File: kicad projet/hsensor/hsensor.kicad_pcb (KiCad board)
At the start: 2 copper layers, 79.5 x 98 mm, 29 parts, among them J2_0 Conn_01x02_Pin, J2_1 Conn_01x02_Pin, J2_2 Conn_01x02_Pin, J3 Conn_01x03_Pin, U1 TLV75801PDBV, U2 TLV75801PDBV, U3 LM358

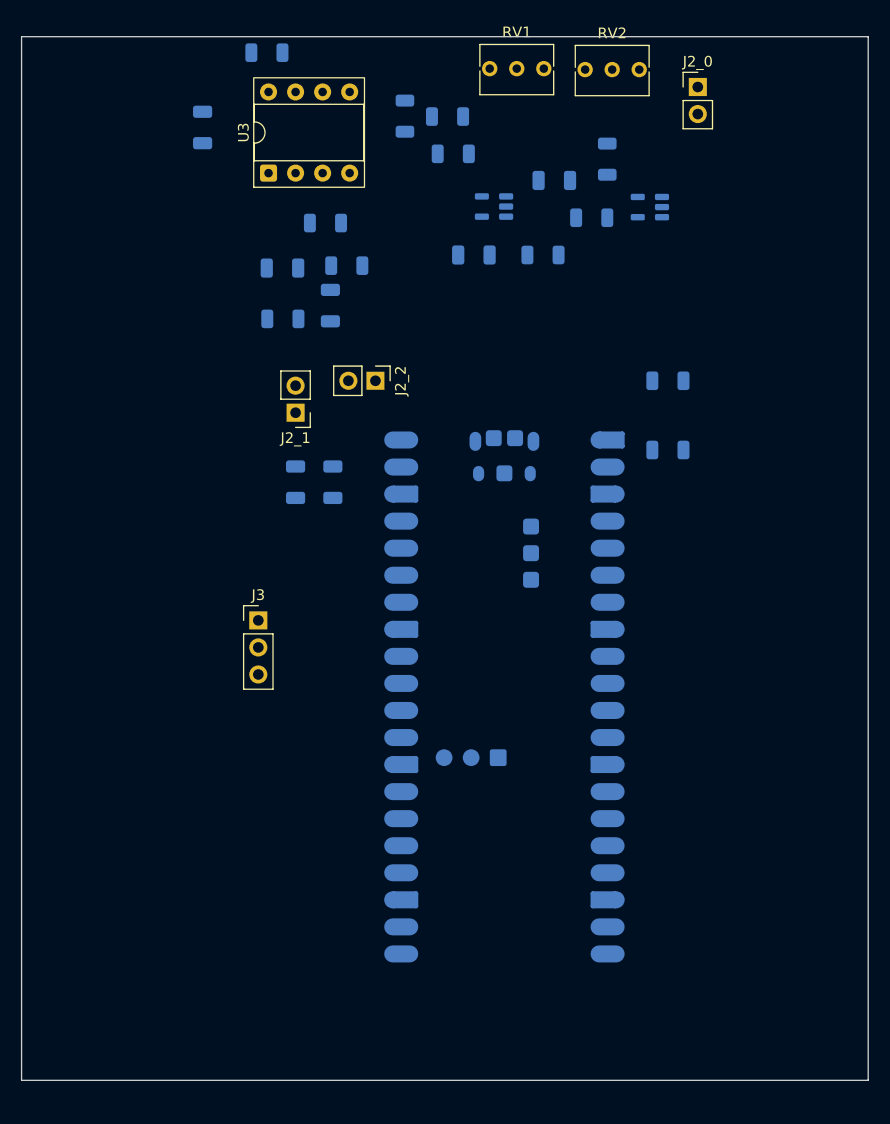
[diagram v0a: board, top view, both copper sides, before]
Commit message: final pcb (i hope)
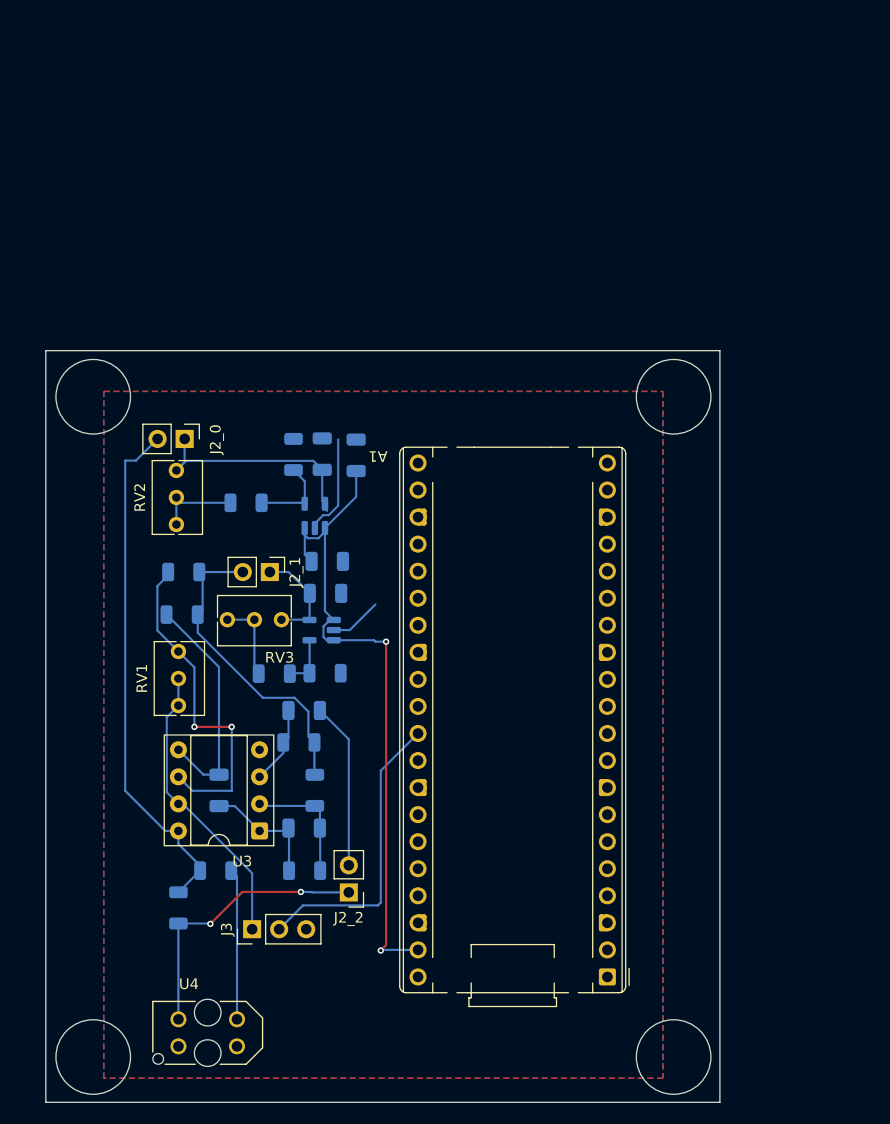
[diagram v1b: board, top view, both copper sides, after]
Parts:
- added U4: TCRT5000, Sensor:OPTO_TCRT5000, F.Cu at (140.8, 142.7)
- A1: footprint Module:RaspberryPi_Pico_W_SMD -> Module:RaspberryPi_Pico_Common_THT; moved to F.Cu
- RV3: value 5e3 -> 5.e3; footprint Resistor_SMD:R_1206_3216Metric -> Potentiometer_THT:Potentiometer_Bourns_3266Y_Vertical; moved to F.Cu
- moved Rsens1 67.5 mm to (138.0, 131.0), turned to -90 degrees
- moved RV1 64.6 mm to (138.0, 106.9), turned to 90 degrees
- moved C3 62.3 mm to (141.8, 120.0)
- moved U3 61.8 mm to (145.6, 123.8), turned to 180 degrees
- moved J2_0 58.4 mm to (138.6, 87.0), turned to -90 degrees
- moved Rsens2 58.0 mm to (141.5, 127.5), turned to 0 degrees
- moved RV2 57.5 mm to (137.8, 89.9), turned to 90 degrees
- moved R6 53.4 mm to (138.3, 103.5)
- moved R4 53.3 mm to (150.8, 120.0), turned to 90 degrees
- moved C2 52.6 mm to (149.8, 123.5)
- moved R5 51.9 mm to (149.8, 127.5)
- moved R11 51.6 mm to (147.0, 109.0)
- moved RV3 49.8 mm to (147.7, 103.9), turned to 0 degrees
- moved J2_2 48.1 mm to (154.0, 129.5), turned to 180 degrees
- moved R7 47.6 mm to (138.5, 99.5), turned to 0 degrees
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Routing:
- net Vsup: track 0.00 -> 63.2 mm, vias 0 -> 2
- net VDD: track 0.00 -> 49.1 mm
- net Net-(U3B--): track 0.00 -> 31.6 mm, vias 0 -> 2
- net VCM: track 0.00 -> 29.3 mm
- net Raspberry_ADC: track 0.00 -> 27.9 mm
- net Net-(J3-Pin_1): track 0.00 -> 27.6 mm
- net Sensor: track 0.00 -> 26.3 mm, vias 0 -> 2
- net Net-(U3B-+): track 0.00 -> 21.8 mm
- net Net-(J2_0-Pin_1): track 0.00 -> 21.7 mm
- net Net-(J2_2-Pin_2): track 0.00 -> 15.7 mm
- net GND: track 0.00 -> 14.7 mm
- net Net-(Rsens2-Pad2): track 0.00 -> 14.2 mm
- net Net-(C2-Pad1): track 0.00 -> 11.1 mm
- net Net-(U3A--): track 0.00 -> 11.0 mm
- net Net-(J2_1-Pin_1): track 0.00 -> 9.73 mm
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- added copper zone on B.Cu, net GND
- added copper zone on F.Cu, net GND
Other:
- board size 79.5 x 98 mm -> 63.3 x 70.6 mm
- board text added: "MARC F GASP V"
- board text added: "PETIT PET"
